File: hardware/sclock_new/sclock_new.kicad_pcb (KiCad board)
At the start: 2 copper layers, 50 parts, among them J1 Conn_02x03_Odd_Even, J2 Conn_FTDI, J3 Screw_Terminal_01x02, J4 Conn_01x03_Male, J5 Screw_Terminal_01x02, Q1 MMBT3904, Q2 MMBT3904, Q3 MMBT3904, Q4 MMBT3906, Q5 MMBT3904, Q6 MMBT3906, Q7 Si2323CDS, SW1 SW_Push, SW2 SW_Push, SW3 SW_SPDT, U1 ATtiny814-SS, U2 DS3231, U3 MAX629, U4 MAX604

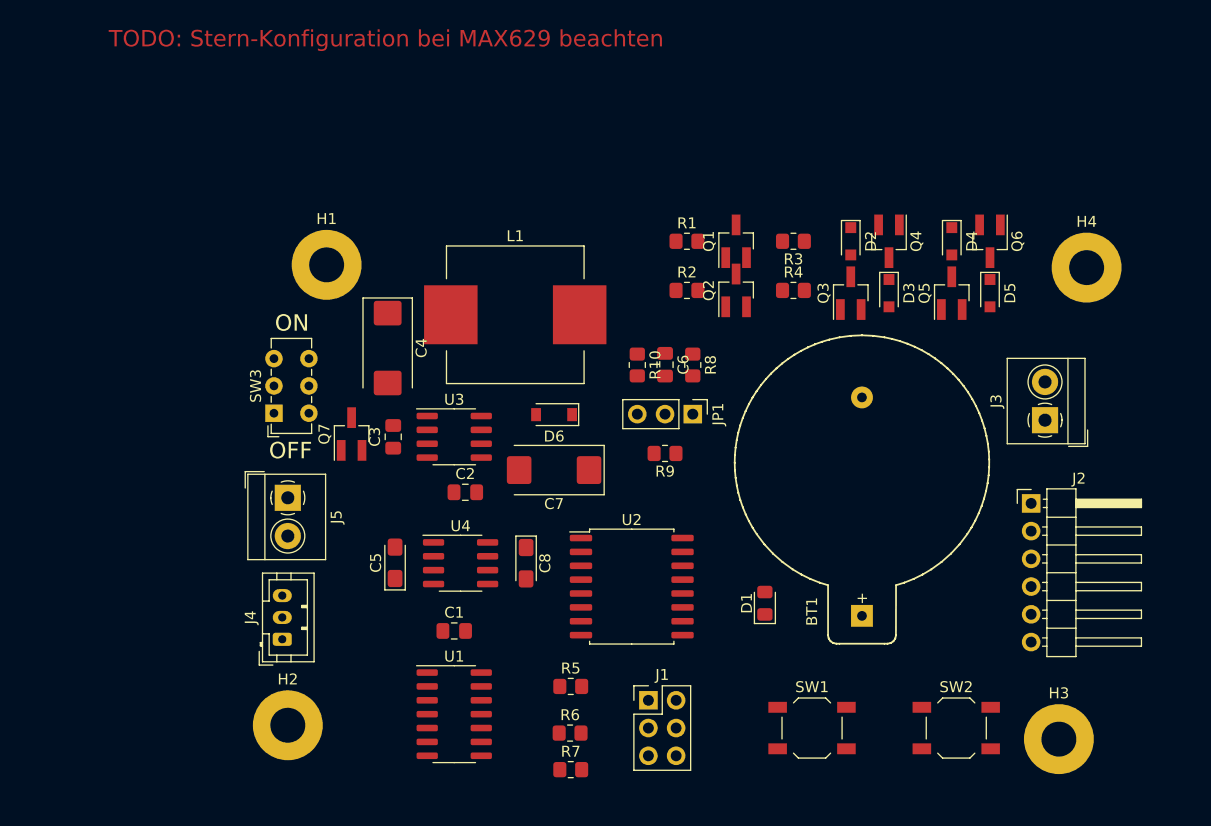
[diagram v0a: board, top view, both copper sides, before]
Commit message: PCB v1.1
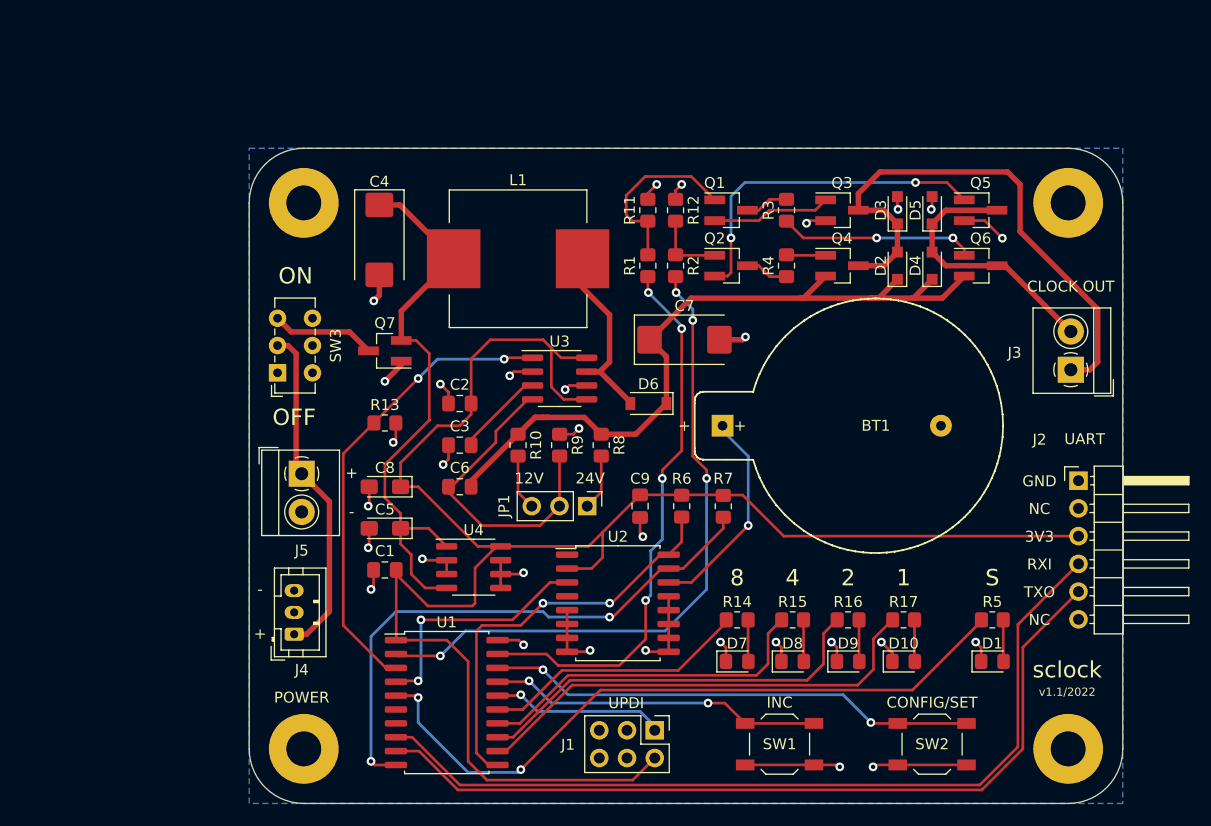
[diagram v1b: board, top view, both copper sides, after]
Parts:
- added C9: 0.1µF, Capacitor_SMD:C_0805_2012Metric_Pad1.18x1.45mm_HandSolder, F.Cu at (145.8, 96.8)
- added D10: LED, LED_SMD:LED_0805_2012Metric_Pad1.15x1.40mm_HandSolder, F.Cu at (169.9, 111.0)
- added D7: LED, LED_SMD:LED_0805_2012Metric_Pad1.15x1.40mm_HandSolder, F.Cu at (154.7, 111.0)
- added D8: LED, LED_SMD:LED_0805_2012Metric_Pad1.15x1.40mm_HandSolder, F.Cu at (159.8, 111.0)
- added D9: LED, LED_SMD:LED_0805_2012Metric_Pad1.15x1.40mm_HandSolder, F.Cu at (164.8, 111.0)
- added R11: 1M, Resistor_SMD:R_0805_2012Metric_Pad1.20x1.40mm_HandSolder, F.Cu at (146.5, 69.7)
- added R12: 1M, Resistor_SMD:R_0805_2012Metric_Pad1.20x1.40mm_HandSolder, F.Cu at (149.0, 69.7)
- added R13: 1M, Resistor_SMD:R_0805_2012Metric_Pad1.20x1.40mm_HandSolder, F.Cu at (122.4, 89.2)
- added R14: 470, Resistor_SMD:R_0805_2012Metric_Pad1.20x1.40mm_HandSolder, F.Cu at (154.7, 107.2)
- added R15: 470, Resistor_SMD:R_0805_2012Metric_Pad1.20x1.40mm_HandSolder, F.Cu at (159.8, 107.2)
- added R16: 470, Resistor_SMD:R_0805_2012Metric_Pad1.20x1.40mm_HandSolder, F.Cu at (164.8, 107.2)
- added R17: 470, Resistor_SMD:R_0805_2012Metric_Pad1.20x1.40mm_HandSolder, F.Cu at (169.9, 107.2)
- Q7: value Si2323CDS -> TSM2323CX
- U1: value ATtiny814-SS -> ATtiny816-S; footprint Package_SO:SOIC-14_3.9x8.7mm_P1.27mm -> Package_SO:SOIC-20W_7.5x12.8mm_P1.27mm
- moved R5 39.1 mm to (178.1, 107.2)
- moved R7 27.9 mm to (153.4, 96.8), turned to -90 degrees
- moved BT1 25.0 mm to (150.9, 89.4), turned to 0 degrees
- moved R6 23.2 mm to (149.6, 96.8), turned to -90 degrees
- moved C6 21.9 mm to (129.3, 95.0), turned to 180 degrees
- moved D1 21.5 mm to (178.1, 111.0), turned to 0 degrees
- moved C7 16.9 mm to (149.9, 81.5), turned to 0 degrees
- moved C8 14.7 mm to (122.4, 95.0), turned to 180 degrees
- moved R10 13.2 mm to (134.6, 91.2)
- moved JP1 12.8 mm to (141.0, 96.8)
- moved R8 11.1 mm to (142.2, 91.2)
- moved U3 11.0 mm to (138.4, 85.1)
- moved C4 9.94 mm to (121.9, 72.4)
- moved R9 9.68 mm to (138.4, 91.2), turned to 90 degrees
- moved D5 9.26 mm to (172.5, 69.7), turned to 90 degrees
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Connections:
- J1 pad 3: Net-(J1-Pad3) -> unconnected-(J1-Pad3)
- J1 pad 4: Net-(J1-Pad4) -> unconnected-(J1-Pad4)
- J1 pad 5: Net-(J1-Pad5) -> unconnected-(J1-Pad5)
- J2 pad 2: Net-(J2-Pad2) -> unconnected-(J2-Pad2)
- J2 pad 6: Net-(J2-Pad6) -> unconnected-(J2-Pad6)
- J4 pad 2: Net-(J4-Pad2) -> unconnected-(J4-Pad2)
- SW3 pad 1: Net-(SW3-Pad1) -> unconnected-(SW3-Pad1)
- U1 pad 10: UPDI -> SDA
- U1 pad 11: CONFIG -> SCL
- U1 pad 12: RESET -> CLED0
- U1 pad 13: CPULSE1 -> CLED1
- U1 pad 14: GND -> CLED2
- U1 pad 6: RXI -> unconnected-(U1-Pad6)
- U1 pad 7: TXO -> unconnected-(U1-Pad7)
- U1 pad 8: SDA -> RXI
- U1 pad 9: SCL -> TXO
- U2 pad 1: Net-(U2-Pad1) -> unconnected-(U2-Pad1)
- U2 pad 4: Net-(U2-Pad4) -> unconnected-(U2-Pad4)
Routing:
- net +3V3: track 0.00 -> 164.8 mm
- net GND: track 0.00 -> 90.5 mm, vias 0 -> 31
- net RXI: track 0.00 -> 79.3 mm
- net TXO: track 0.00 -> 77.0 mm
- net +24V: track 0.00 -> 70.4 mm
- net LED: track 0.00 -> 63.6 mm, vias 0 -> 2
- net CPULSE2: track 0.00 -> 60.6 mm, vias 0 -> 4
- net VCC: track 0.00 -> 52.9 mm
- net SDA: track 0.00 -> 51.0 mm, vias 0 -> 2
- net CPULSE1: track 0.00 -> 50.9 mm, vias 0 -> 4
- net COUT1: track 0.00 -> 50.4 mm
- net RESET: track 0.00 -> 45.1 mm, vias 0 -> 2
- net SHDN: track 0.00 -> 43.1 mm, vias 0 -> 2
- net CLED0: track 0.00 -> 42.0 mm
- net CLED1: track 0.00 -> 37.2 mm
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- added copper zone on B.Cu, net GND
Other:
- board outline added: 80 x 60 mm
- net class Default removed
- board text added: "+"
- board text added: "-"
- board text added: "1"
- board text added: "12V"
- board text added: "2"
- board text added: "24V"
- board text added: "3V3"
- board text added: "4"
- board text added: "8"
- board text added: "CLOCK OUT"
- board text added: "CONFIG/SET"
- board text added: "GND"
- board text added: "INC"
- board text added: "NC"
- board text added: "POWER"
- board text added: "RXI"
- board text added: "S"
- board text added: "TXO"
- board text added: "UART"
- board text added: "UPDI"
- board text added: "buckket.org/sclock"
- board text added: "sclock"
- board text added: "v1.1/2022"
- board text removed: "TODO: Stern-Konfiguration bei MAX629 beachten"
